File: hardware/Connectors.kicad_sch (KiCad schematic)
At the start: 3 parts, among them J2 Conn_02x20_Odd_Even, U1 AS222-35PN-933

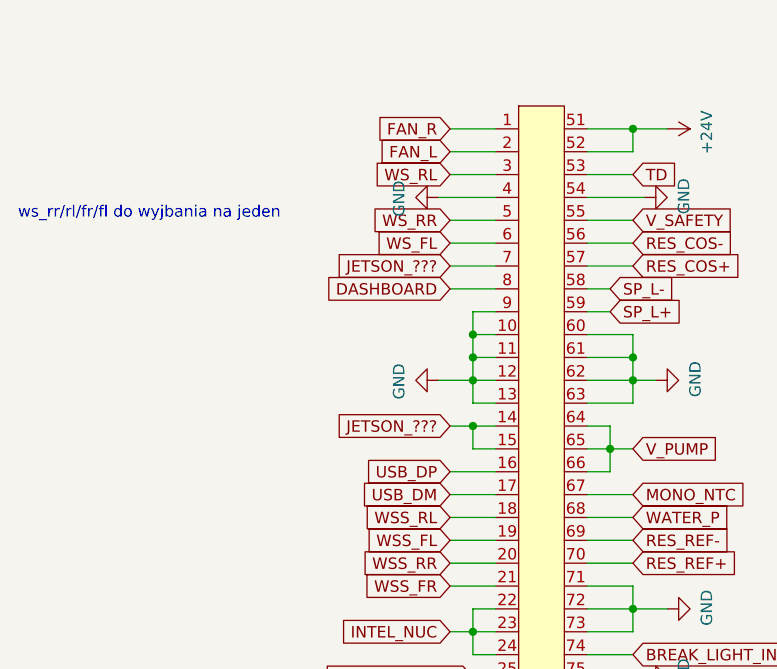
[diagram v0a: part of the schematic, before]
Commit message: jolo
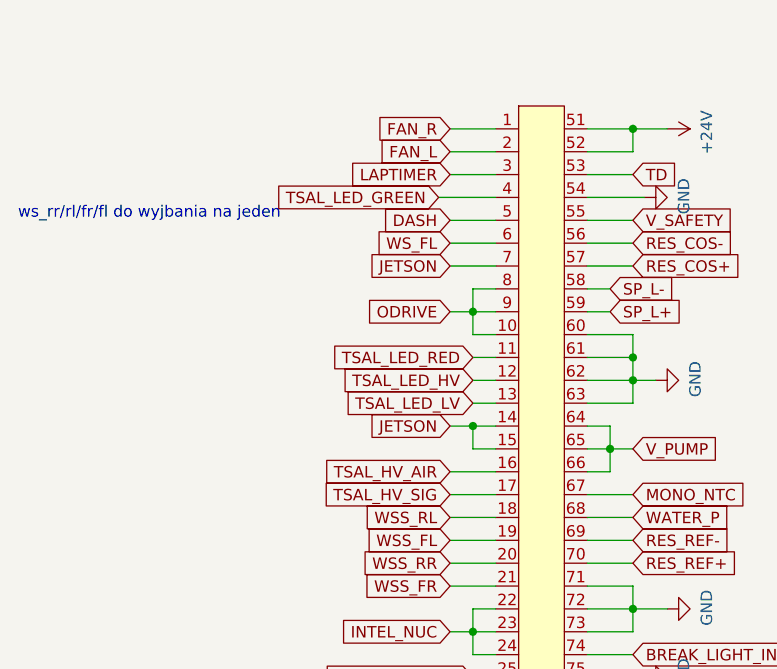
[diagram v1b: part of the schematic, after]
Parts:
- U1: footprint AS222-35PN-933C:AS222-35PN-933C-ver3-drill_0.72_size_1.02 -> Autosport:AS222-35PN-933C-ver4-drill_0.72_size_1.02
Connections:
- net GND: no longer U1.10, U1.11, U1.12, U1.13, U1.4, U1.9
- net USB_DM: no longer U1.17
- net USB_DP: no longer U1.16
- net DASHBOARD renamed ODRIVE
- net ODRIVE: now also U1.10, U1.9
- net JETSON_??? renamed JETSON
- net WS_RL renamed LAPTIMER
- net WS_RR renamed DASH
- new net TSAL_HV_AIR: U1.16
- new net TSAL_HV_SIG: U1.17
- new net TSAL_LED_GREEN: U1.4
- new net TSAL_LED_HV: U1.12
- new net TSAL_LED_LV: U1.13
- new net TSAL_LED_RED: U1.11
